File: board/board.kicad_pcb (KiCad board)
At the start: 2 copper layers, 41.1 x 31.5 mm, 23 parts, among them J1 Conn_01x05, J2 Conn_ARM_JTAG_SWD_20, J3 Conn_01x10, P1 USB_C_Plug_USB2.0, SW1 RST, SW2 BOOT, U1 FT232RL, U2 AMS1117-3.3

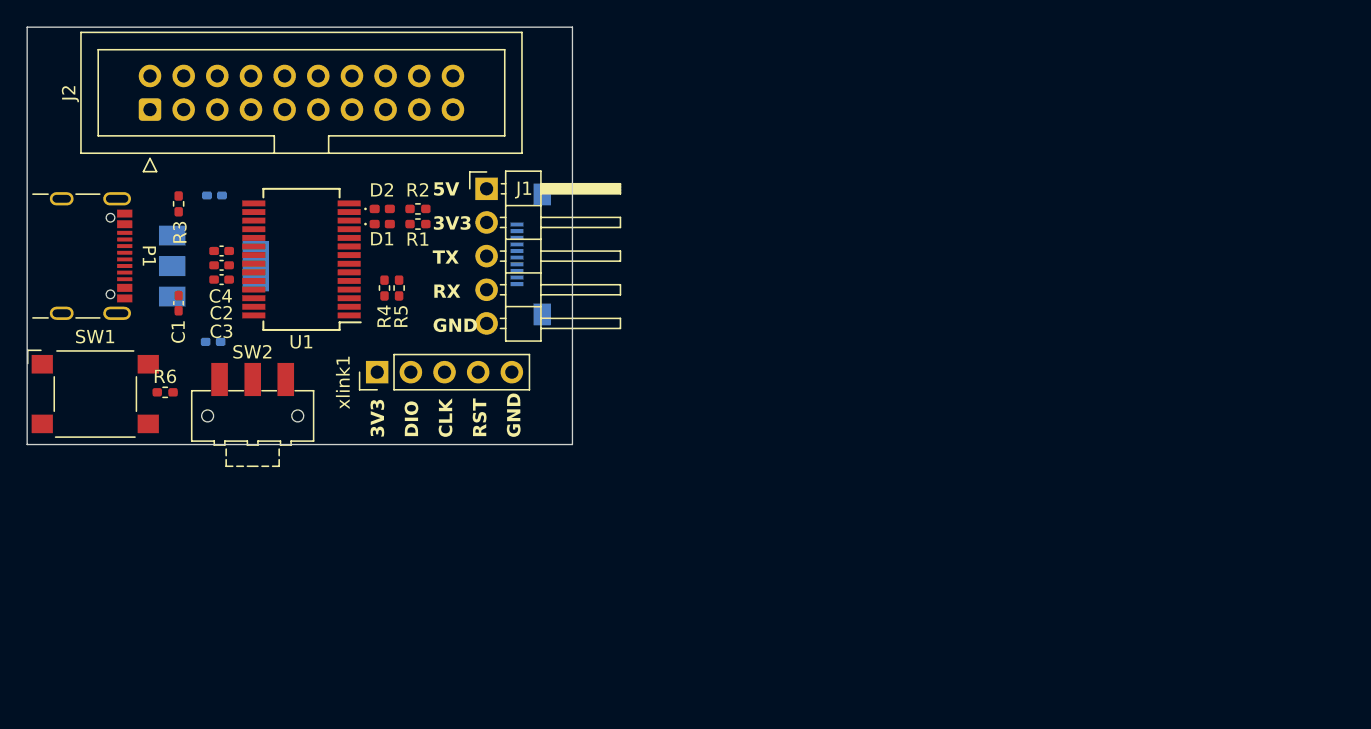
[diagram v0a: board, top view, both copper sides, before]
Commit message: feat(bsp/usb-ttl/debug): pcb layer
aa
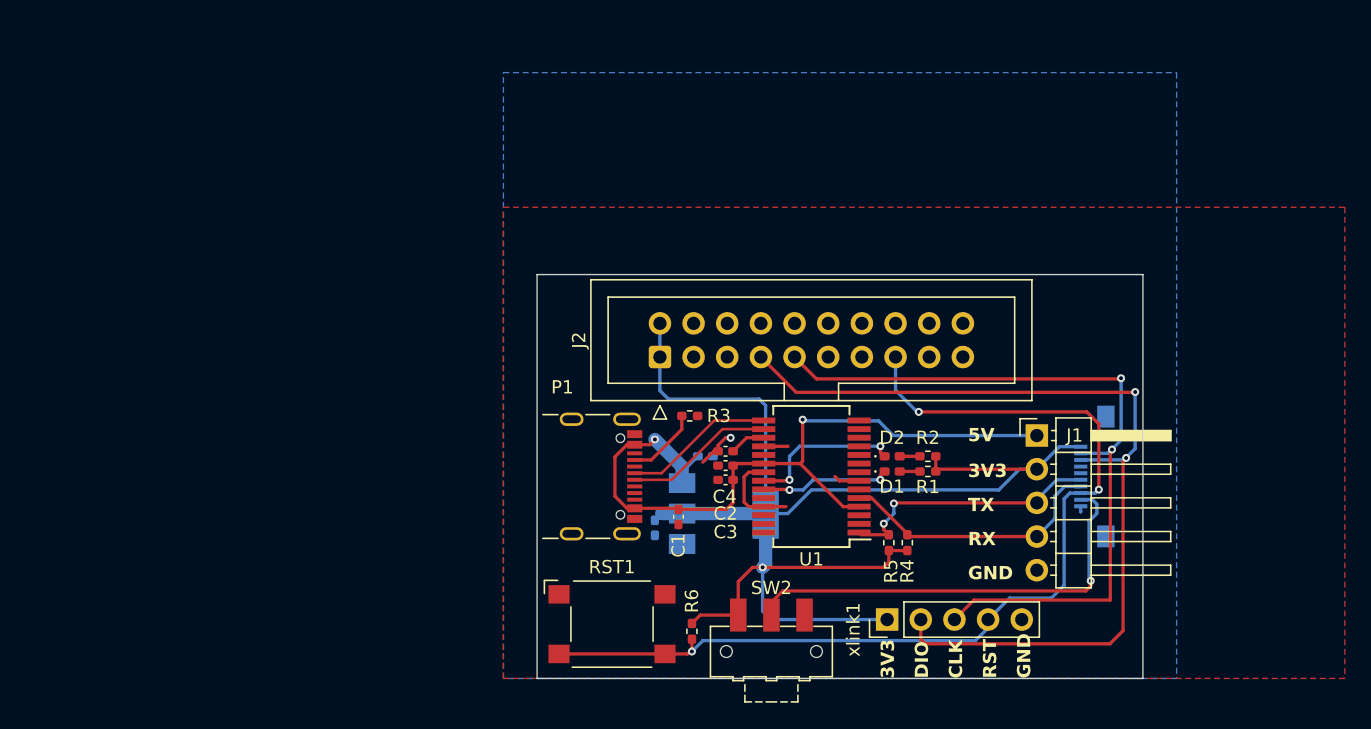
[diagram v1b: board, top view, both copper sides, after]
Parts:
- moved J3 45.7 mm to (169.1, 111.8)
- moved J1 45.5 mm to (164.7, 108.7)
- moved R4 43.9 mm to (154.9, 116.8)
- moved R6 43.7 mm to (138.7, 123.4), turned to -90 degrees
- moved SW2 43.0 mm to (144.7, 125.0)
- moved R1 42.8 mm to (156.5, 111.4)
- moved R2 42.8 mm to (156.5, 110.2)
- moved U2 42.8 mm to (141.1, 114.6)
- moved D1 42.8 mm to (153.8, 111.4)
- moved D2 42.8 mm to (153.8, 110.2)
- moved xlink1 42.8 mm to (153.4, 122.6)
- moved J2 42.8 mm to (136.3, 102.7)
- moved RST1 42.7 mm to (132.7, 122.9)
- moved C5 42.0 mm to (139.7, 110.2), turned to 0 degrees
- moved P1 41.9 mm to (130.7, 111.8)
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- renumbered SW1 to RST1
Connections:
- J3 pad 1: unconnected-(J3-Pin_1-Pad1) -> +3.3V
- J3 pad 2: unconnected-(J3-Pin_2-Pad2) -> /SWCLK
- J3 pad 3: +3.3V -> /SWDIO
- J3 pad 4: /BOOT -> unconnected-(J3-Pin_4-Pad4)
- J3 pad 5: /RST -> unconnected-(J3-Pin_5-Pad5)
- J3 pad 8: /SWCLK -> /RST
- J3 pad 9: /SWDIO -> /BOOT
- R6 pad 2: Net-(R6-Pad2) -> /RST
- RST1 pad 2: Net-(R6-Pad2) -> /RST
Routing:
- net +3.3V: track 0.00 -> 102.6 mm, vias 0 -> 1
- net /RST: track 0.00 -> 74.6 mm, vias 0 -> 3
- net /SWDIO: track 0.00 -> 68.2 mm, vias 0 -> 2
- net +5V: track 0.00 -> 58.0 mm, vias 0 -> 2
- net /SWCLK: track 0.00 -> 56.9 mm, vias 0 -> 2
- net /BOOT: track 0.00 -> 33.4 mm, vias 0 -> 1
- net /RX: track 0.00 -> 20.5 mm
- net /TX: track 0.00 -> 20.1 mm, vias 0 -> 2
- net GND: track 0.00 -> 14.2 mm, vias 0 -> 1
- net /RXLED: track 0.00 -> 11.8 mm, vias 0 -> 2
- net /D+: track 0.00 -> 11.4 mm
- net /D-: track 0.00 -> 11.3 mm
- net /TXLED: track 0.00 -> 9.91 mm, vias 0 -> 2
- net Net-(P1-CC): track 0.00 -> 5.53 mm
- net /3V3: track 0.00 -> 2.73 mm
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- added copper zone on B.Cu, net GND
- added copper zone on F.Cu, net GND
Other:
- board size 41.1 x 31.5 mm -> 45.7 x 30.5 mm
